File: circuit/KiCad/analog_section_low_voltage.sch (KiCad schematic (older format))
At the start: 41 parts, among them J6 Screw_Terminal_01x09, J7 Screw_Terminal_01x09, U11 LM7332, U12 CPC1114N, U13 CPC1114N, U14 LM321LV

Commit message: qe
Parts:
- U14: PartNo (none) -> 595-LM321LVIDBVR; Supplier (none) -> Mouser
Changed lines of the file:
@@
 F 2 "Package_TO_SOT_SMD:SOT-23-5" H 1850 3850 50  0001 C CNN
 F 3 "http://www.ti.com/lit/ds/symlink/lm321.pdf" H 1850 3850 50  0001 C CNN
+F 4 "595-LM321LVIDBVR" H 1850 3850 50  0001 C CNN "PartNo"
+F 5 "Mouser" H 1850 3850 50  0001 C CNN "Supplier"
 	1    1850 3850
 	1    0    0    -1

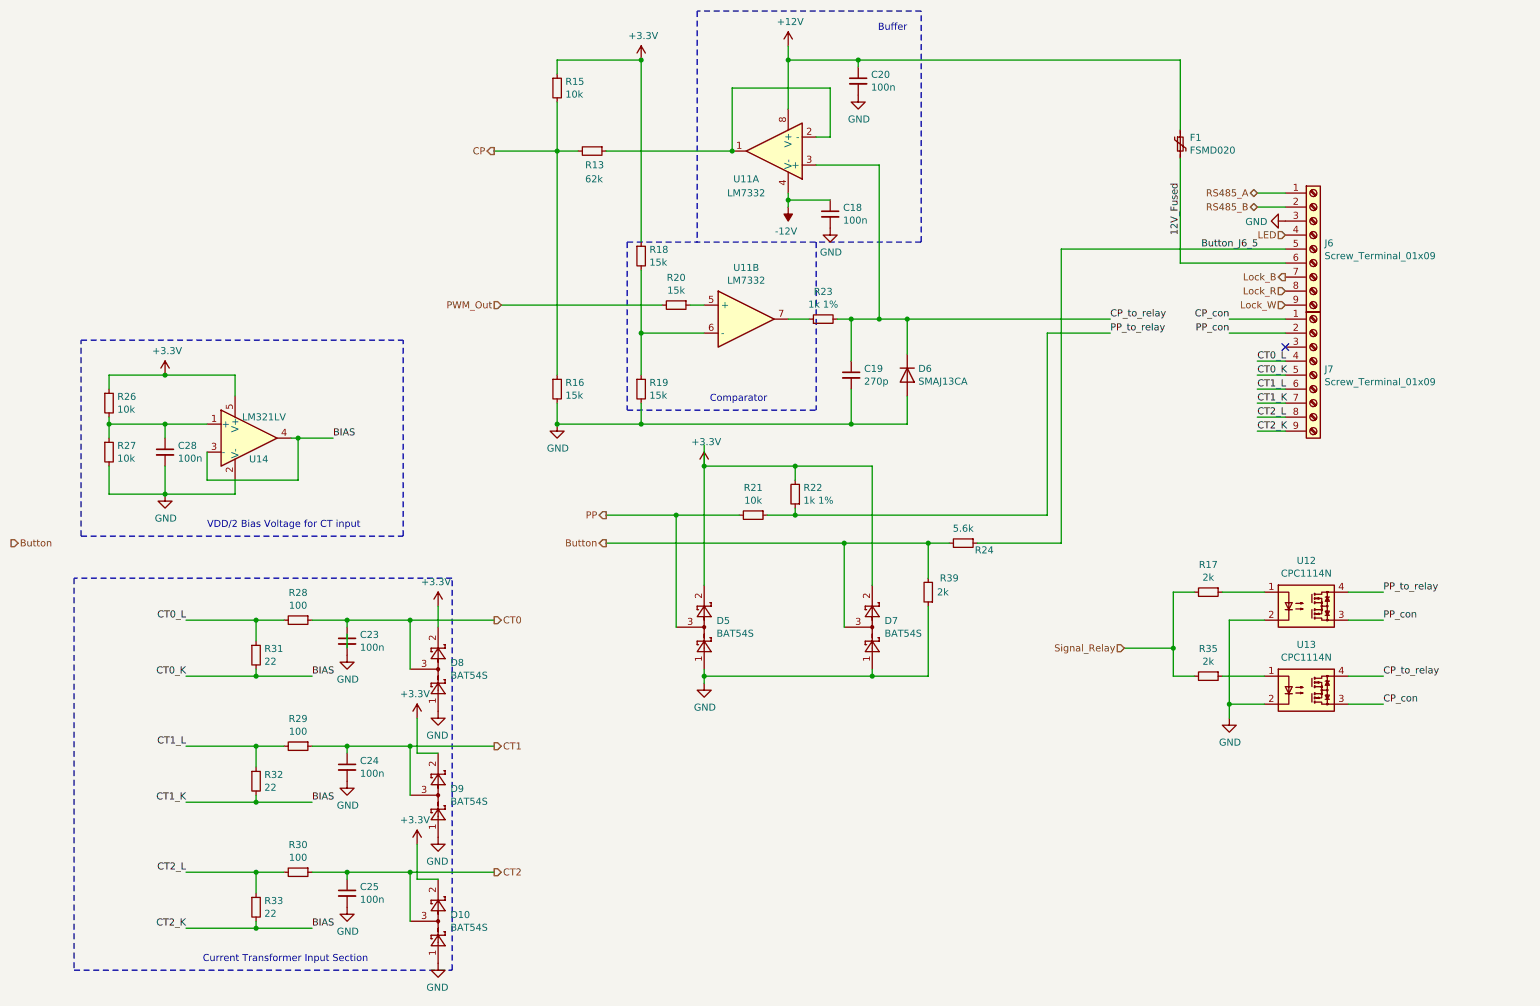
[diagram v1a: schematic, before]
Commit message: qe
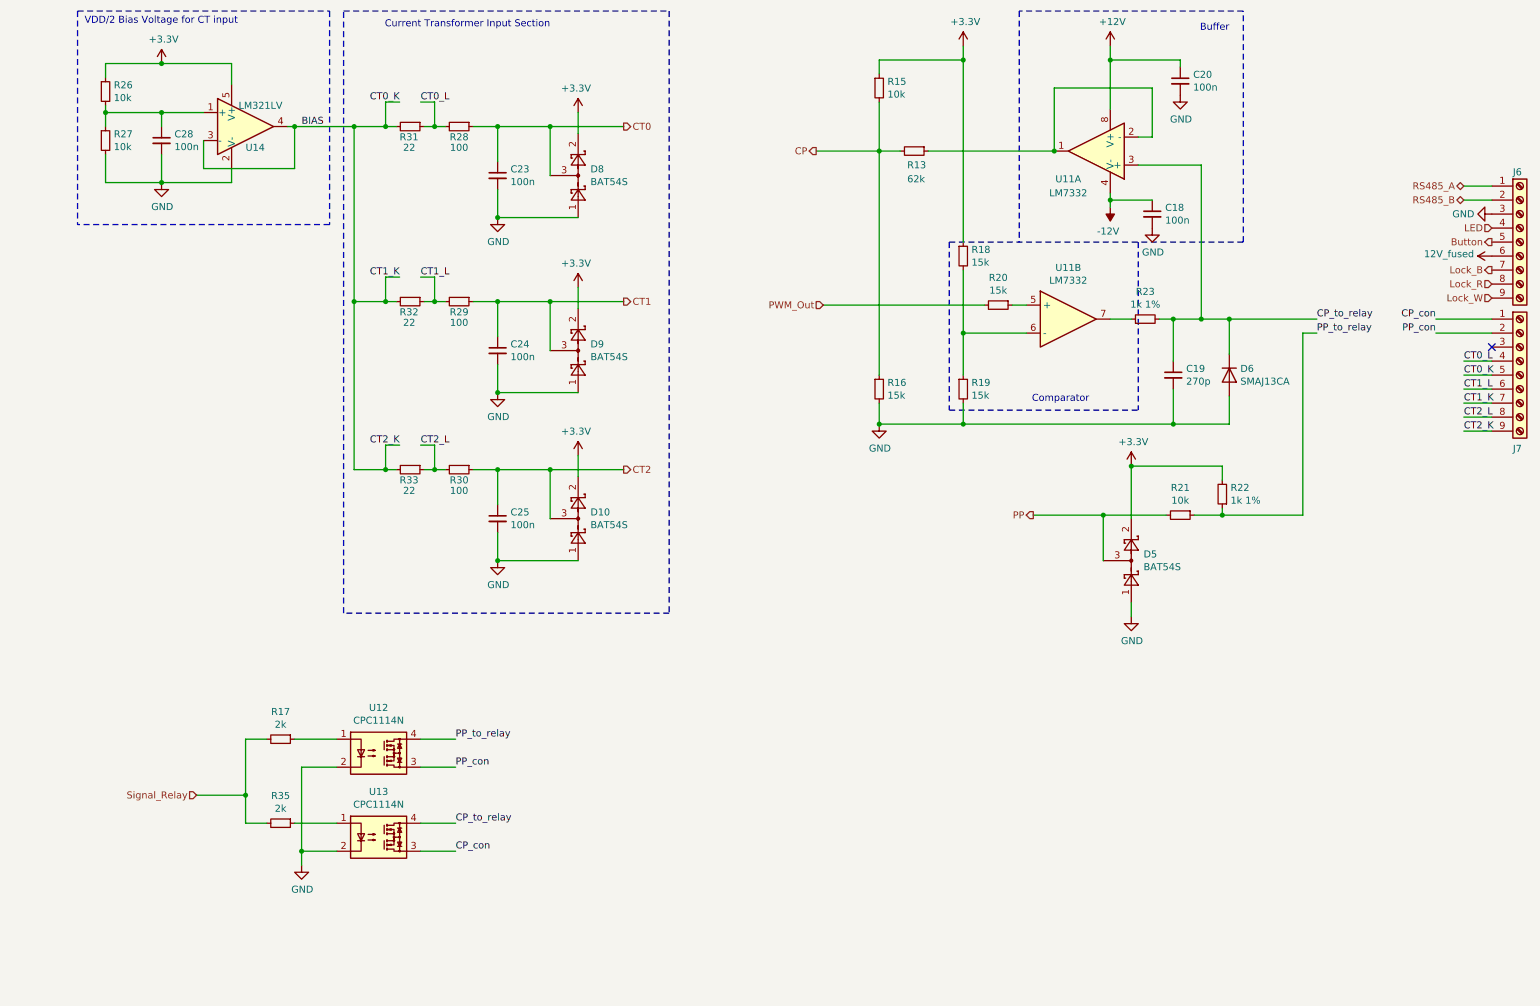
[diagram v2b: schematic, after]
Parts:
- removed D7: BAT54S, Package_TO_SOT_SMD:SOT-23_Handsoldering, symbol Diode:BAT54S
- removed F1: FSMD020, Fuse:Fuse_1812_4532Metric_Pad1.30x3.40mm_HandSolder, symbol Device:Polyfuse_Small
- removed R24: 5.6k, Resistor_SMD:R_0603_1608Metric_Pad1.05x0.95mm_HandSolder, symbol Device:R_Small
- removed R39: 2k, Resistor_SMD:R_0603_1608Metric_Pad1.05x0.95mm_HandSolder, symbol Device:R_Small
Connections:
- net Button_J6_5 is gone; now on net Button: J6.5 (Pin_5)
- net 12V_Fused renamed 12V_fused
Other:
- moved on the sheet: C18, C19, C20, C23, C24, C25, C28, D10, D5, D6, D8, D9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
